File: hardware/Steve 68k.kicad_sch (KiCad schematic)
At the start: 45 parts, among them IC1 MC68008FN8, J1 Conn_02x32_Odd_Even, J2 Serial 1, J3 Serial 2, J4 Conn_01x03_Male, SW1 Reset, U1 74LS32, U2 28C256, U3 GAL16V8, U4 74HC04, U5 MC68681FN, U7 AS6C4008-55PCN, U8 Max705, X1 CXO_DIP8, X2 1.8432 Mhz

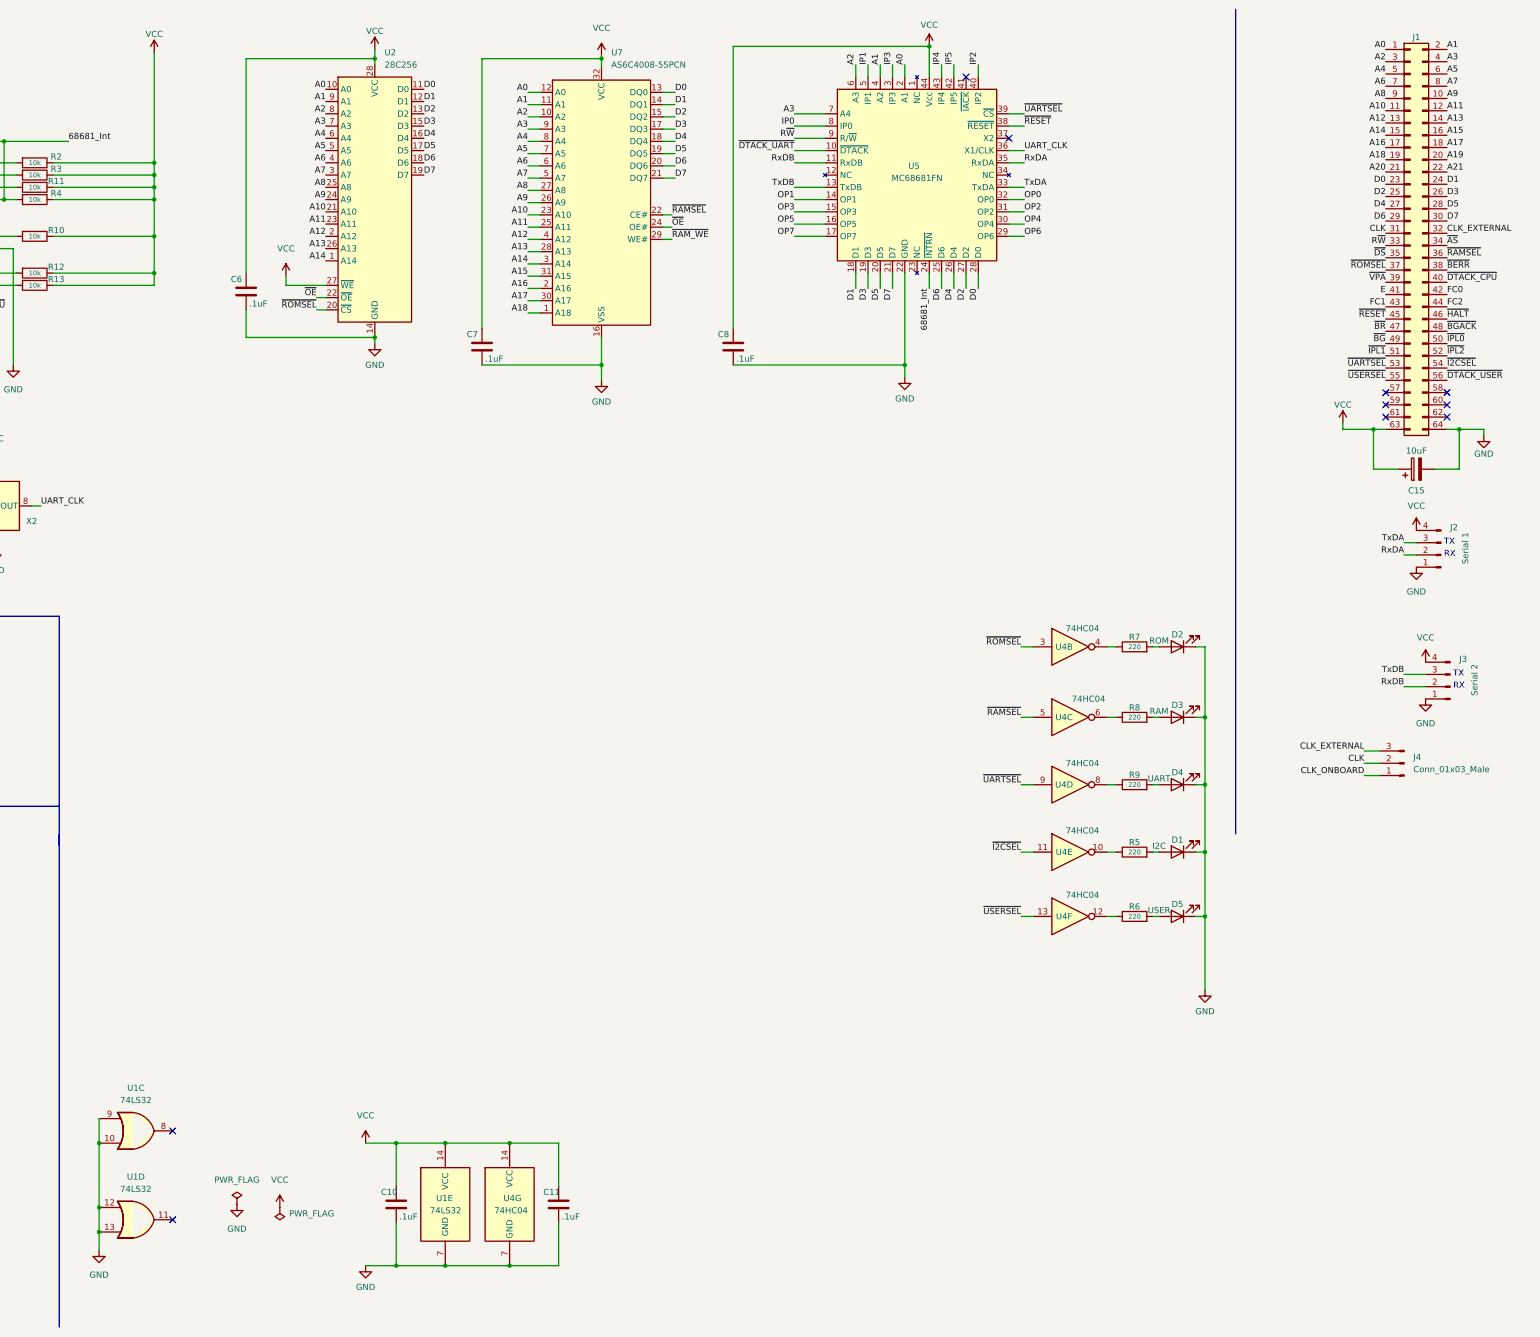
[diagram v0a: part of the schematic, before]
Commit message: More GAL and glue logic stuff
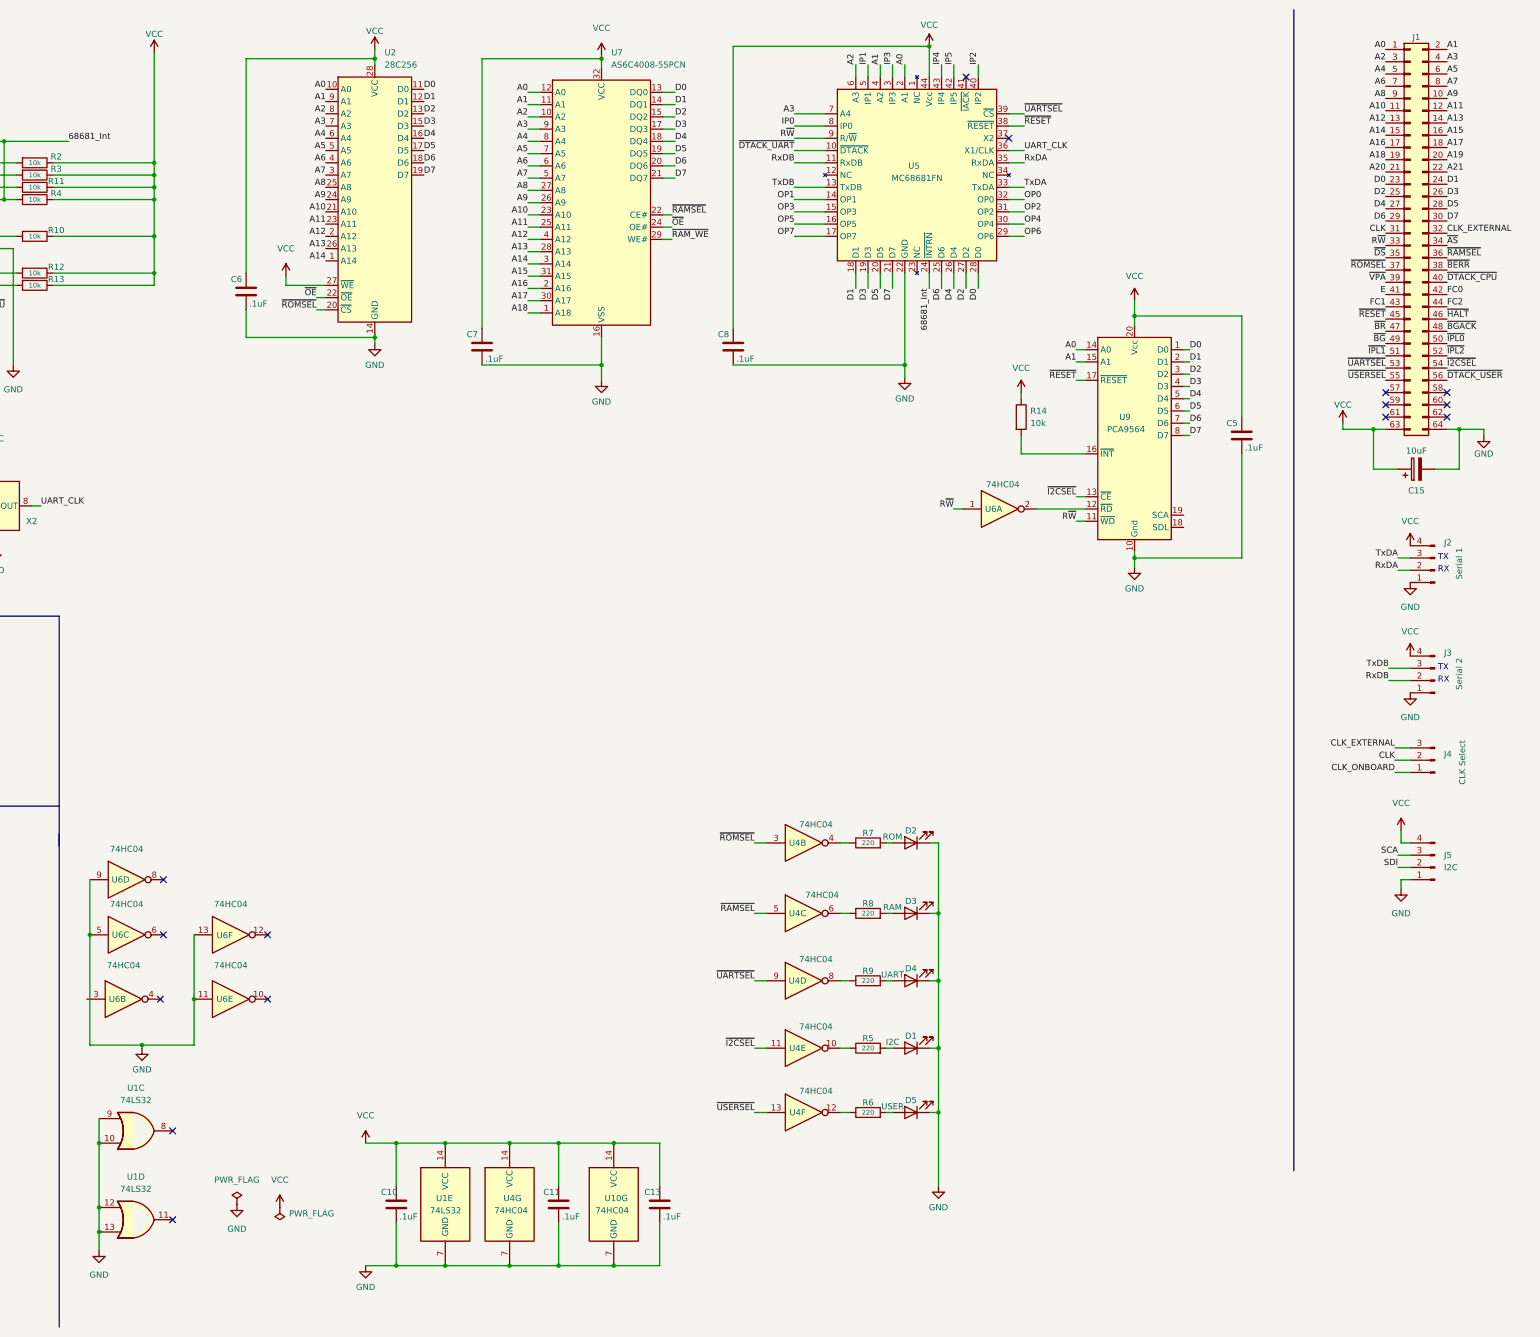
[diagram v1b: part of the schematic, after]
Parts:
- added C13, C5: .1uF, Capacitor_SMD:C_0603_1608Metric, symbol Device:C
- added J5: I2C, symbol Connector:Conn_01x04_Male
- added R14: 10k, symbol Device:R
- added U10, U6: 74HC04, symbol 74xx:74HC04
- added U9: PCA9564, symbol mc68k:PCA9564
- J4: value Conn_01x03_Male -> CLK Select
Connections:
- net A0: now also U9.14 (A0)
- net A1: now also U9.15 (A1)
- net D0: now also U9.1 (D0)
- net D1: now also U9.2 (D1)
- net D2: now also U9.3 (D2)
- net D3: now also U9.4 (D3)
- net D4: now also U9.5 (D4)
- net D5: now also U9.6 (D5)
- net D6: now also U9.7 (D6)
- net D7: now also U9.8 (D7)
- net GND: now also C13.2, C5.2, J5.1 (Pin_1), U10.7 (GND), U6.11, U6.13, U6.5, U6.9, U9.10 (Gnd)
- net R~{W}: now also U6.1, U9.11 (~{WD})
- net VCC: now also C13.1, C5.1, J5.4 (Pin_4), R14.1, U10.14 (VCC), U9.20 (Vcc)
- net ~{I2CSEL}: now also U9.13 (~{CE})
- net ~{RESET}: now also U9.17 (~{RESET})
- new net: U6.2, U9.12 (~{RD})
- new net: R14.2, U9.16 (~{INT})
- new net SCA: J5.3 (Pin_3)
- new net SDl: J5.2 (Pin_2)
- no-connect marks 18 -> 23
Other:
- moved on the sheet: D1, D2, D3, D4, D5, J2, J3, J4, R5, R6, R7, R8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
